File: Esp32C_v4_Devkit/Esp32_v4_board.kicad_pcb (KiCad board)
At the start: 2 copper layers, 28 x 54.5 mm, 34 parts, among them J1 USB_CON8, J2 Conn_01x19_Male, J3 Conn_01x19_Male, Q1 SS8O5O-G, Q2 SS8O5O-G, SW1 SW_Push, SW2 SW_Push, U1 CP2102N-A01-GQFN28, U2 AMS117_3.3

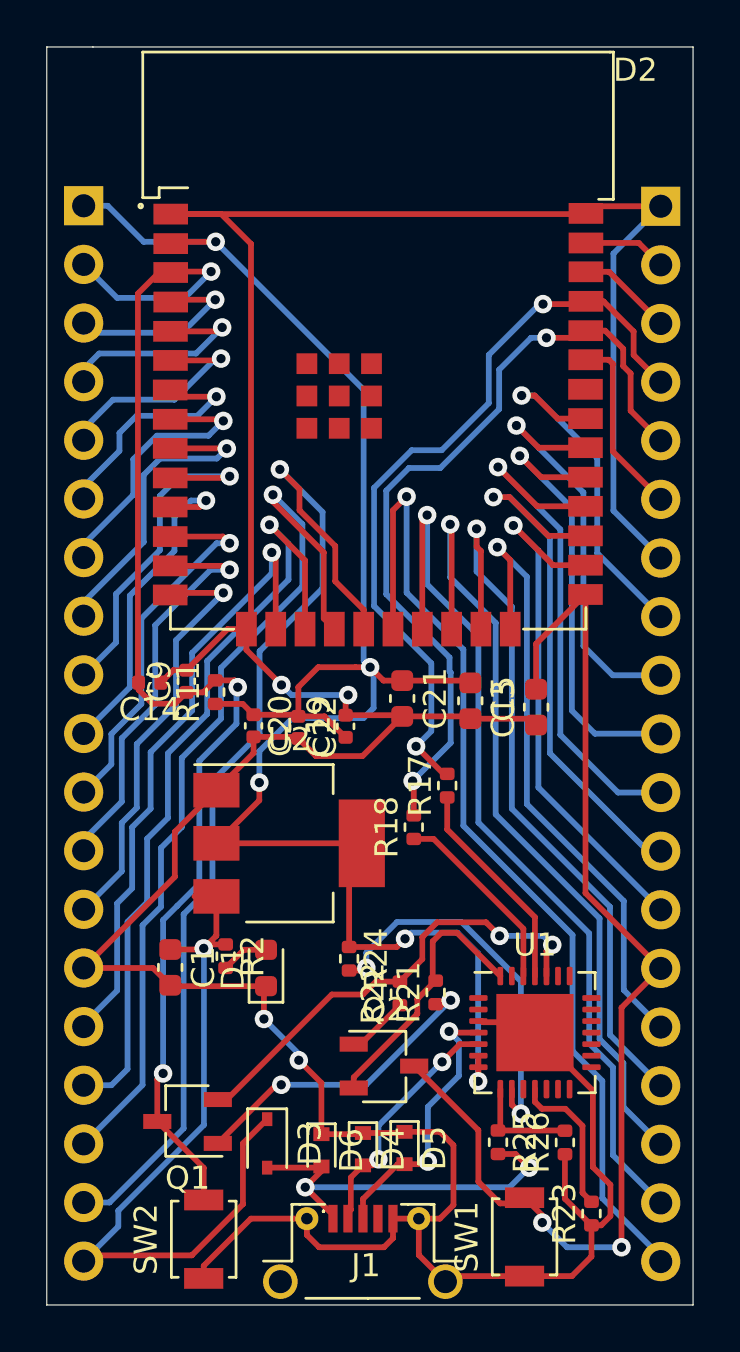
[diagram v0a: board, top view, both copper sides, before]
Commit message: Routing and components placement
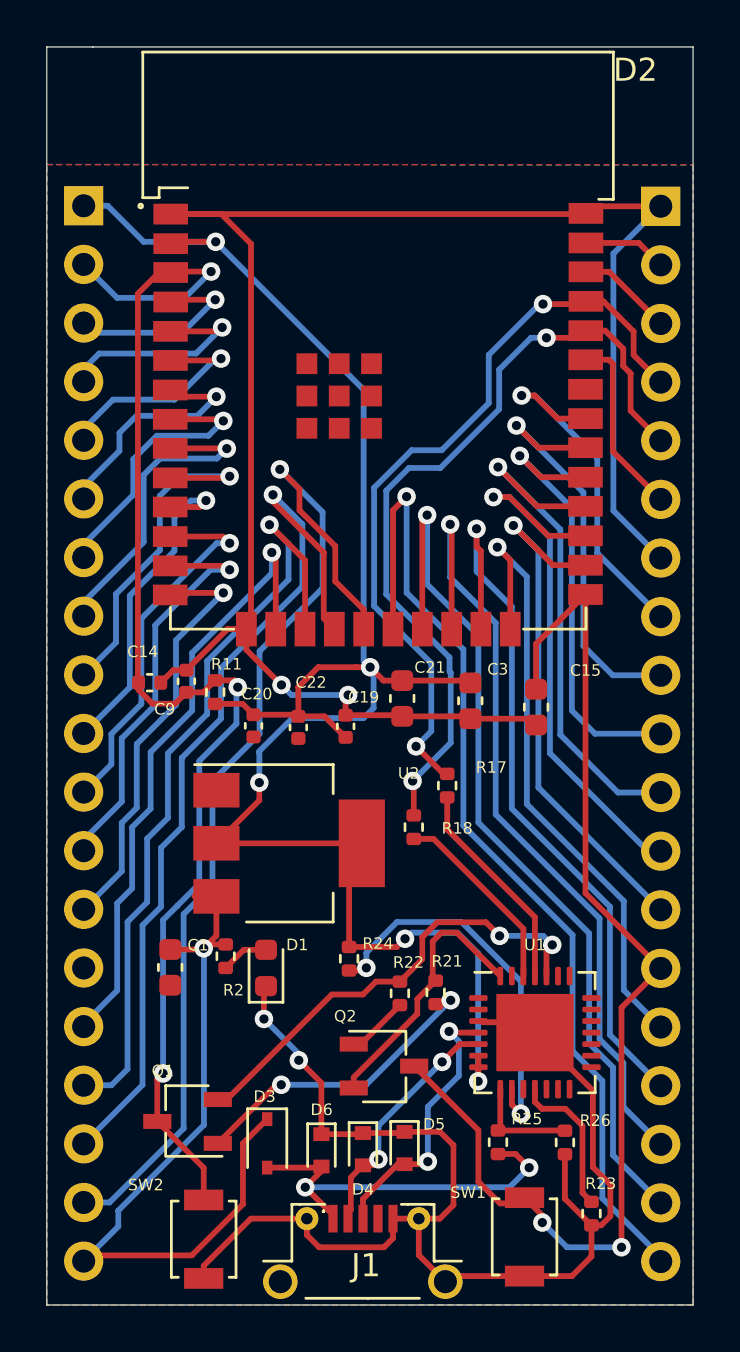
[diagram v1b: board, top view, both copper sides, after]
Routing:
- net GND: track 166.3 -> 137.5 mm
- added copper zone on B.Cu, net GND
- added copper zone on F.Cu, net GND
